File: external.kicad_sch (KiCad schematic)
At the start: 5 parts, among them CN3 STE_I2C_QT, M1 Motor_Servo, M2 Motor_Servo

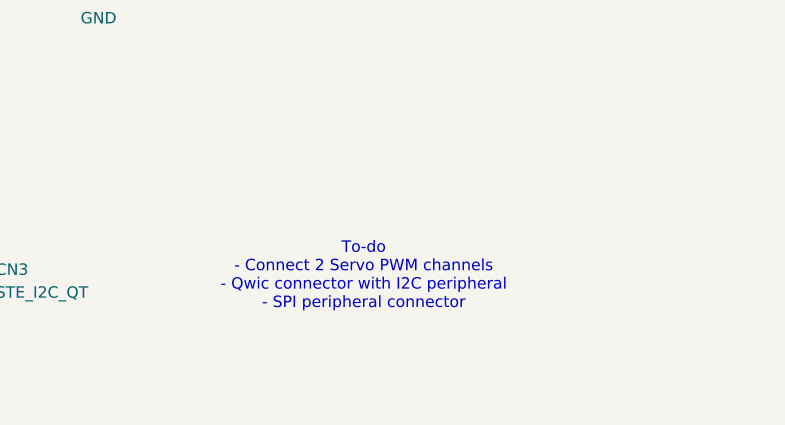
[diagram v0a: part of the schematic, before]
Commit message: Current progress on externals
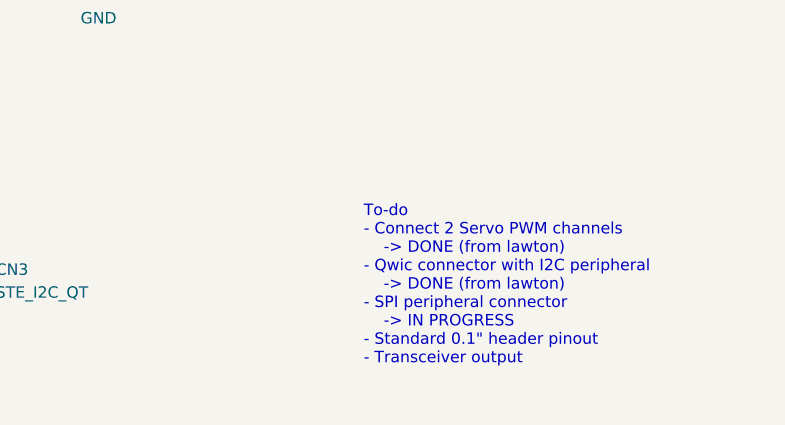
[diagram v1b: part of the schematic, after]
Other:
- note added: "To-do - Connect 2 Servo PWM channels -> DONE (from lawton) - Qwic connector with I2C peripheral -> DONE (from lawton) - SPI peripheral connector -> IN PROGRESS - Standard 0.1" header pinout - Transceiver output"
- note removed: "To-do - Connect 2 Servo PWM channels - Qwic connector with I2C peripheral - SPI peripheral connector"
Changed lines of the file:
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@@
 	(generator_version "9.0")
 	(paper "A4")
-	(text "To-do \n- Connect 2 Servo PWM channels \n- Qwic connector with I2C peripheral\n- SPI peripheral connector\n\n"
+	(text "To-do \n- Connect 2 Servo PWM channels \n	-> DONE (from lawton)\n- Qwic connector with I2C peripheral\n	-> DONE (from lawton)\n- SPI peripheral connector\n	-> IN PROGRESS\n- Standard 0.1\" header pinout\n- Transceiver output\n"
 		(exclude_from_sim no)
 		(at 123.444 88.138 0)
@@
 				(size 1.27 1.27)
 			)
+			(justify left)
 		)
 	)
